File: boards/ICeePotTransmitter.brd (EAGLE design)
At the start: 100 x 80 mm, 8 parts, among them IC1 RFPIC12F675

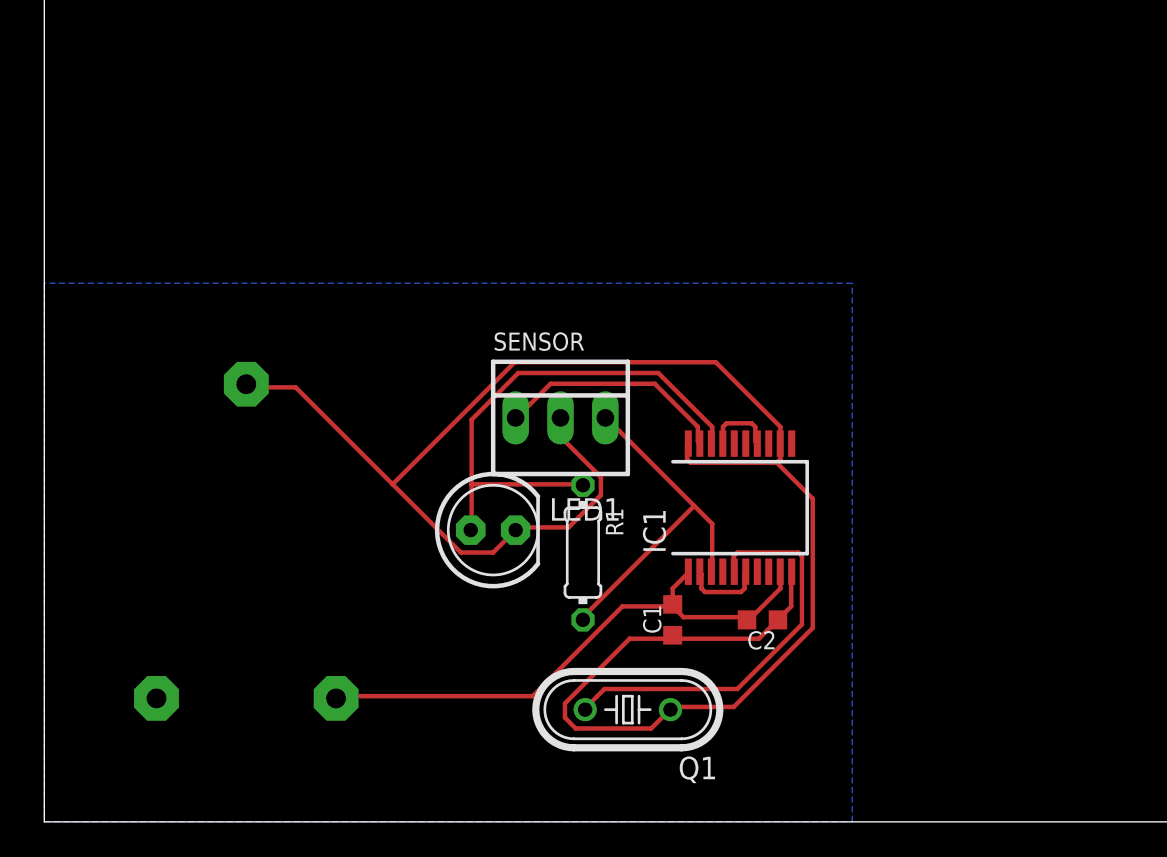
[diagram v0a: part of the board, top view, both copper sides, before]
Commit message: put all the downloaded files into directories
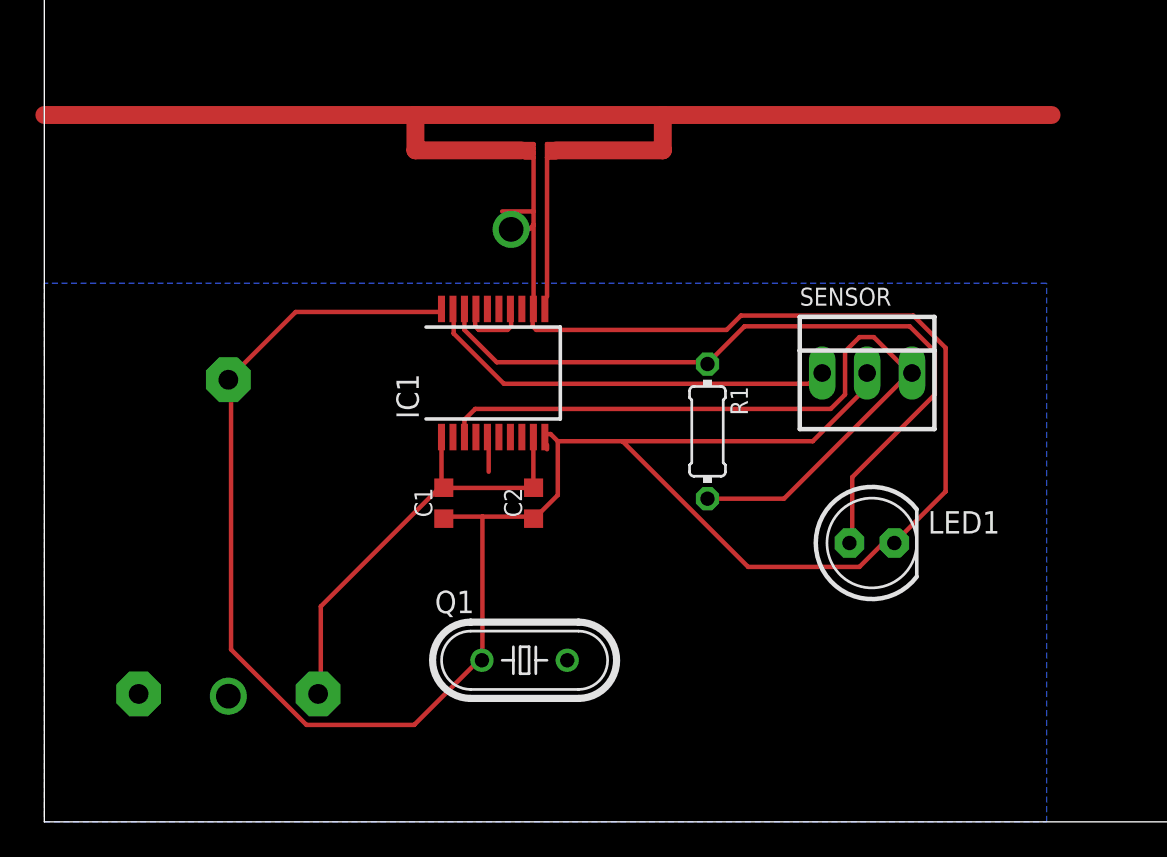
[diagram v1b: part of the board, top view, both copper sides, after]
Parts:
- moved LED1 21.4 mm to (46.8, 15.8)
- moved SENSOR 17.5 mm to (46.6, 25.4)
- moved IC1 15.9 mm to (25.4, 25.4)
- moved C1 14.5 mm to (22.6, 18.0)
- moved C2 14.5 mm to (27.7, 18.0), turned to 90 degrees
- moved R1 9.83 mm to (37.5, 22.1)
- moved Q1 6.48 mm to (27.2, 9.14), turned to 0 degrees
- moved G1 1.05 mm to (10.4, 18.0)
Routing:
- net N$11: track 0.00 -> 73.0 mm
- net N$7: track 110.1 -> 142.2 mm
- net N$4: track 20.3 -> 44.9 mm
- net N$6: track 23.1 -> 2.03 mm
- net N$3: track 29.5 -> 43.0 mm
- net N$10: track 0.00 -> 13.0 mm
- net N$1: track 13.1 -> 23.7 mm
- net N$9: track 0.00 -> 9.65 mm
- net N$5: track 31.7 -> 25.7 mm
- net N$8: track 4.55 -> 0.00 mm
